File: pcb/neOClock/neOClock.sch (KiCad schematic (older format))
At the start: 46 parts, among them J1 Barrel_Jack, J2 Conn_01x04, J3 Conn_01x04, J4 Conn_01x04, J5 ATECC508A, Q1 2n2222a, Q2 2n2222a, SW1 G71Y, SW2 G71Y, SW3 G71Y, U1 DCDC_LM2596, U2 AMS1117, U3 ESP32_dev_30p, U4 SA15-11GWA, U5 SA15-11GWA, U6 SAA1064, U7 SA15-11GWA, U8 SA15-11GWA

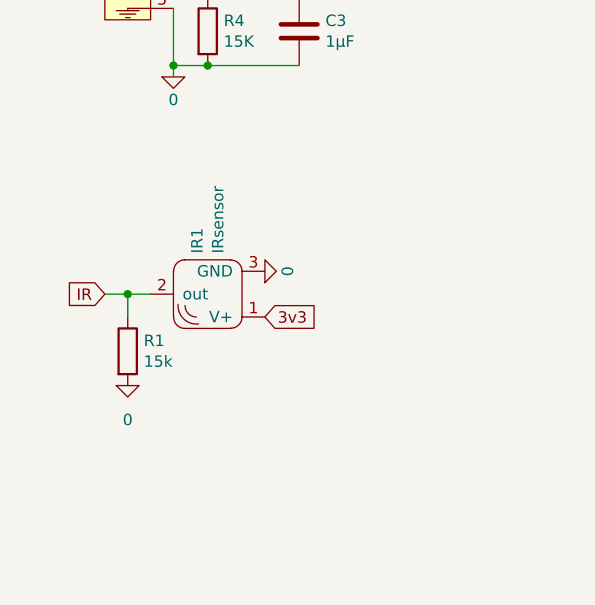
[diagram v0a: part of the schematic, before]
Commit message: update
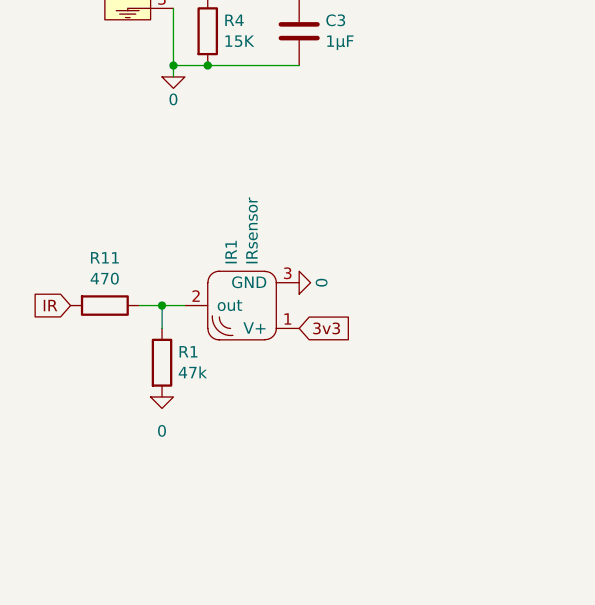
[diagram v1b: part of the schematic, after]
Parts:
- added R11: 470, Resistor_SMD:R_0805_2012Metric_Pad1.20x1.40mm_HandSolder, symbol Device:R
- R1: value 15k -> 47k
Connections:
- net IR: now also R11.2; no longer IR1.2 (out), R1.1
- new net: IR1.2 (out), R1.1, R11.1
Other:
- moved on the sheet: IR1, R1
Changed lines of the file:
@@
 L neosensor_addon:IRsensor IR1
 U 1 1 60A834AB
-P 1300 3700
-F 0 "IR1" V 1346 3522 50  0000 R CNN
-F 1 "IRsensor" V 1255 3522 50  0000 R CNN
-F 2 "neosensor_addon:IRsensor_TH_and_smd" H 1300 3700 50  0001 C CIN
-F 3 "" H 1300 3700 50  0001 C CNN
-	1    1300 3700
+P 1450 3750
+F 0 "IR1" V 1496 3572 50  0000 R CNN
+F 1 "IRsensor" V 1405 3572 50  0000 R CNN
+F 2 "neosensor_addon:IRsensor_TH_and_smd" H 1450 3750 50  0001 C CIN
+F 3 "" H 1450 3750 50  0001 C CNN
+	1    1450 3750
 	-1   0    0    1
 $EndComp
@@
 L pspice:0 #GND0111
 U 1 1 60A9911E
-P 1550 3600
-F 0 "#GND0111" H 1550 3500 50  0001 C CNN
-F 1 "0" H 1550 3500 50  0000 C CNN
-F 2 "" H 1550 3600 50  0001 C CNN
-F 3 "~" H 1550 3600 50  0001 C CNN
-	1    1550 3600
+P 1700 3650
+F 0 "#GND0111" H 1700 3550 50  0001 C CNN
+F 1 "0" H 1700 3550 50  0000 C CNN
+F 2 "" H 1700 3650 50  0001 C CNN
+F 3 "~" H 1700 3650 50  0001 C CNN
+	1    1700 3650
 	0    -1   -1   0
 $EndComp
@@
 Text GLabel 4150 1550 2    50   Input ~ 0
 SCL
-Text GLabel 1550 3800 2    50   Input ~ 0
+Text GLabel 1700 3850 2    50   Input ~ 0
 3v3
 $Comp
@@
 Text GLabel 1750 2350 2    50   Input ~ 0
 Push_3
-Text GLabel 850  3700 0    50   Input ~ 0
+Text GLabel 700  3750 0    50   Input ~ 0
 IR
 Text GLabel 3400 6850 2    50   Input ~ 0
@@
 L Device:R R1
 U 1 1 61383ACF
-P 950 3950
-F 0 "R1" H 1020 3996 50  0000 L CNN
-F 1 "15k" H 1020 3905 50  0000 L CNN
-F 2 "Resistor_SMD:R_0805_2012Metric_Pad1.20x1.40mm_HandSolder" V 880 3950 50  0001 C CNN
-F 3 "~" H 950 3950 50  0001 C CNN
-	1    950  3950
+P 1100 4000
+F 0 "R1" H 1170 4046 50  0000 L CNN
+F 1 "47k" H 1170 3955 50  0000 L CNN
+F 2 "Resistor_SMD:R_0805_2012Metric_Pad1.20x1.40mm_HandSolder" V 1030 4000 50  0001 C CNN
+F 3 "~" H 1100 4000 50  0001 C CNN
+	1    1100 4000
 	1    0    0    -1
 $EndComp
@@
 L pspice:0 #GND0125
 U 1 1 61384771
-P 950 4100
-F 0 "#GND0125" H 950 4000 50  0001 C CNN
-F 1 "0" H 950 3950 50  0000 C CNN
-F 2 "" H 950 4100 50  0001 C CNN
-F 3 "~" H 950 4100 50  0001 C CNN
-	1    950  4100
-	1    0    0    -1
-$EndComp
-Wire Wire Line
-	850  3700 950  3700
-Wire Wire Line
-	950  3700 950  3800
-Connection ~ 950  3700
-Wire Wire Line
-	950  3700 1050 3700
+P 1100 4150
+F 0 "#GND0125" H 1100 4050 50  0001 C CNN
+F 1 "0" H 1100 4000 50  0000 C CNN
+F 2 "" H 1100 4150 50  0001 C CNN
+F 3 "~" H 1100 4150 50  0001 C CNN
+	1    1100 4150
+	1    0    0    -1
+$EndComp
+Wire Wire Line
+	1000 3750 1100 3750
+Wire Wire Line
+	1100 3750 1100 3850
+Connection ~ 1100 3750
+Wire Wire Line
+	1100 3750 1200 3750
 Wire Wire Line
 	3300 6850 3300 6950
@@
 NoConn ~ 8125 1700
 NoConn ~ 10150 1700
+$Comp
+L Device:R R11
+U 1 1 60C98695
+P 850 3750
+F 0 "R11" V 643 3750 50  0000 C CNN
+F 1 "470" V 734 3750 50  0000 C CNN
+F 2 "Resistor_SMD:R_0805_2012Metric_Pad1.20x1.40mm_HandSolder" V 780 3750 50  0001 C CNN
+F 3 "~" H 850 3750 50  0001 C CNN
+	1    850  3750
+	0    1    1    0
+$EndComp
 Wire Bus Line
 	9950 1100 9950 2950

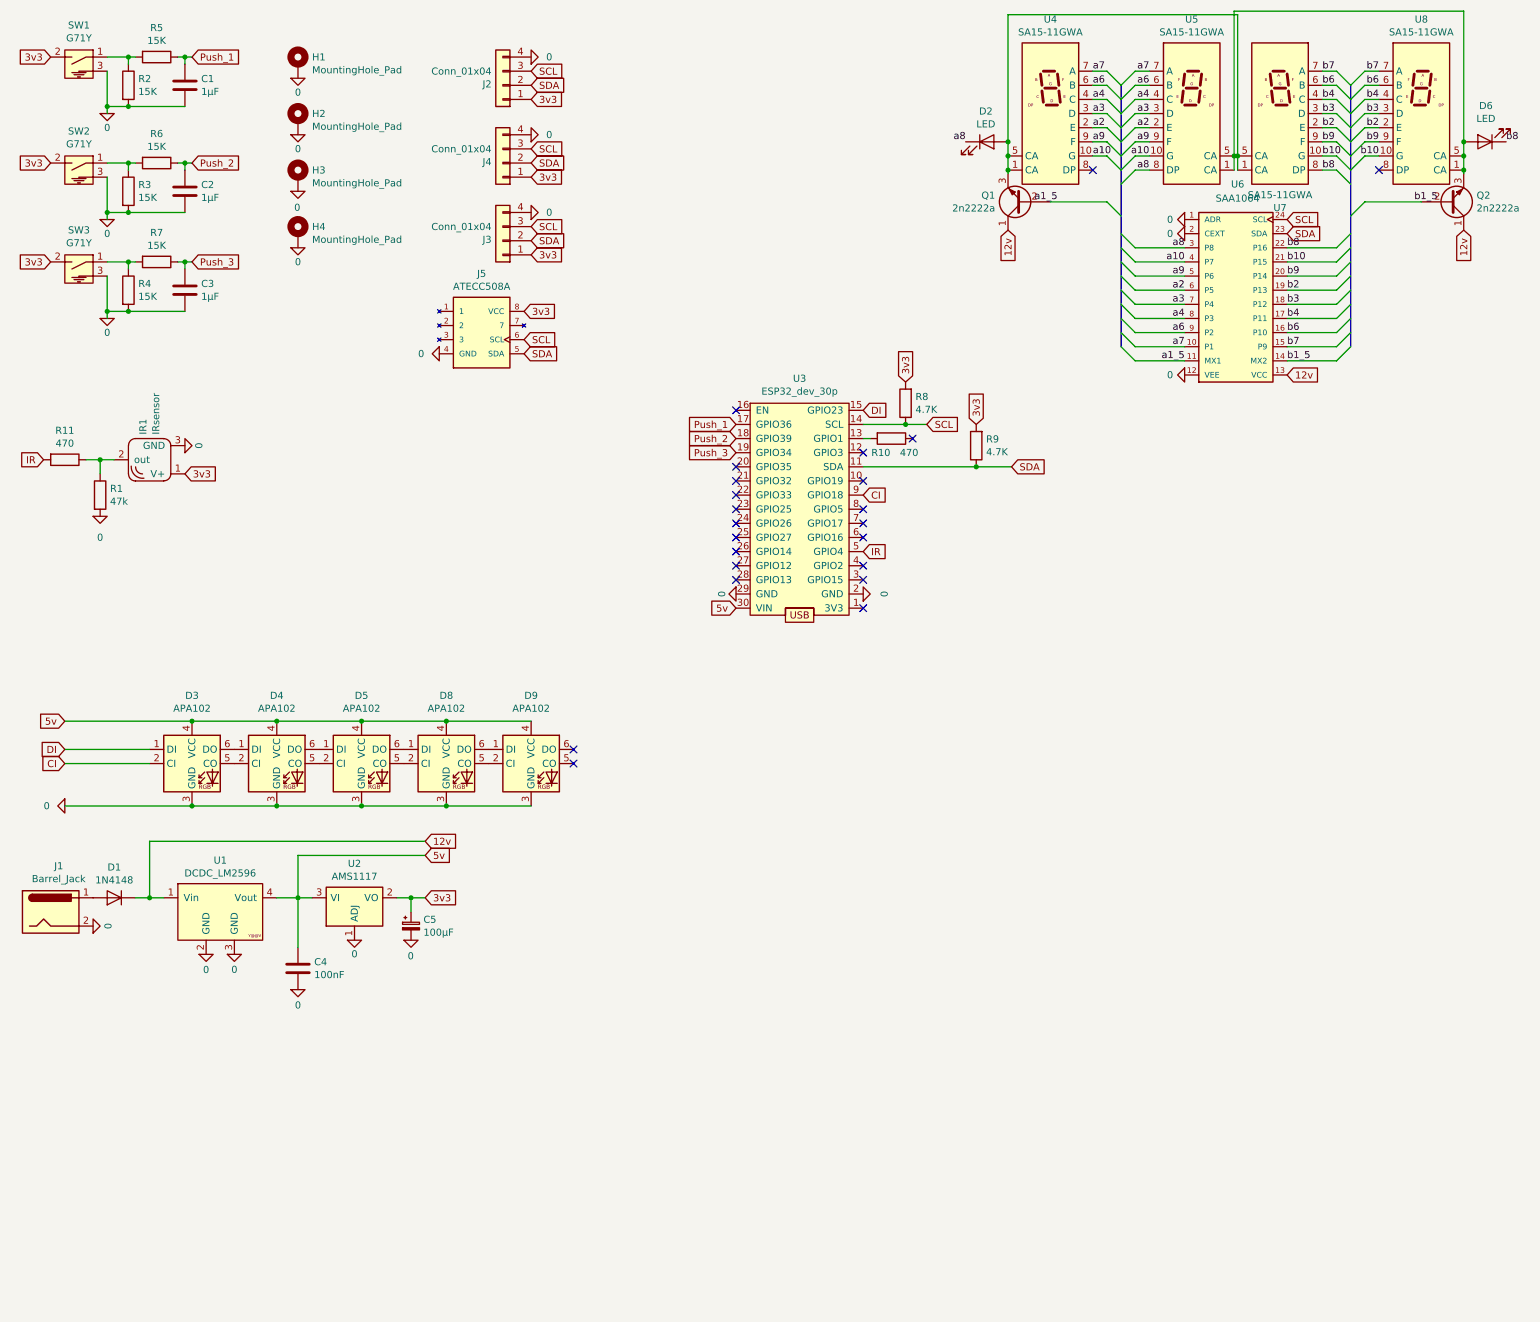
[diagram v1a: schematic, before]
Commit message: update
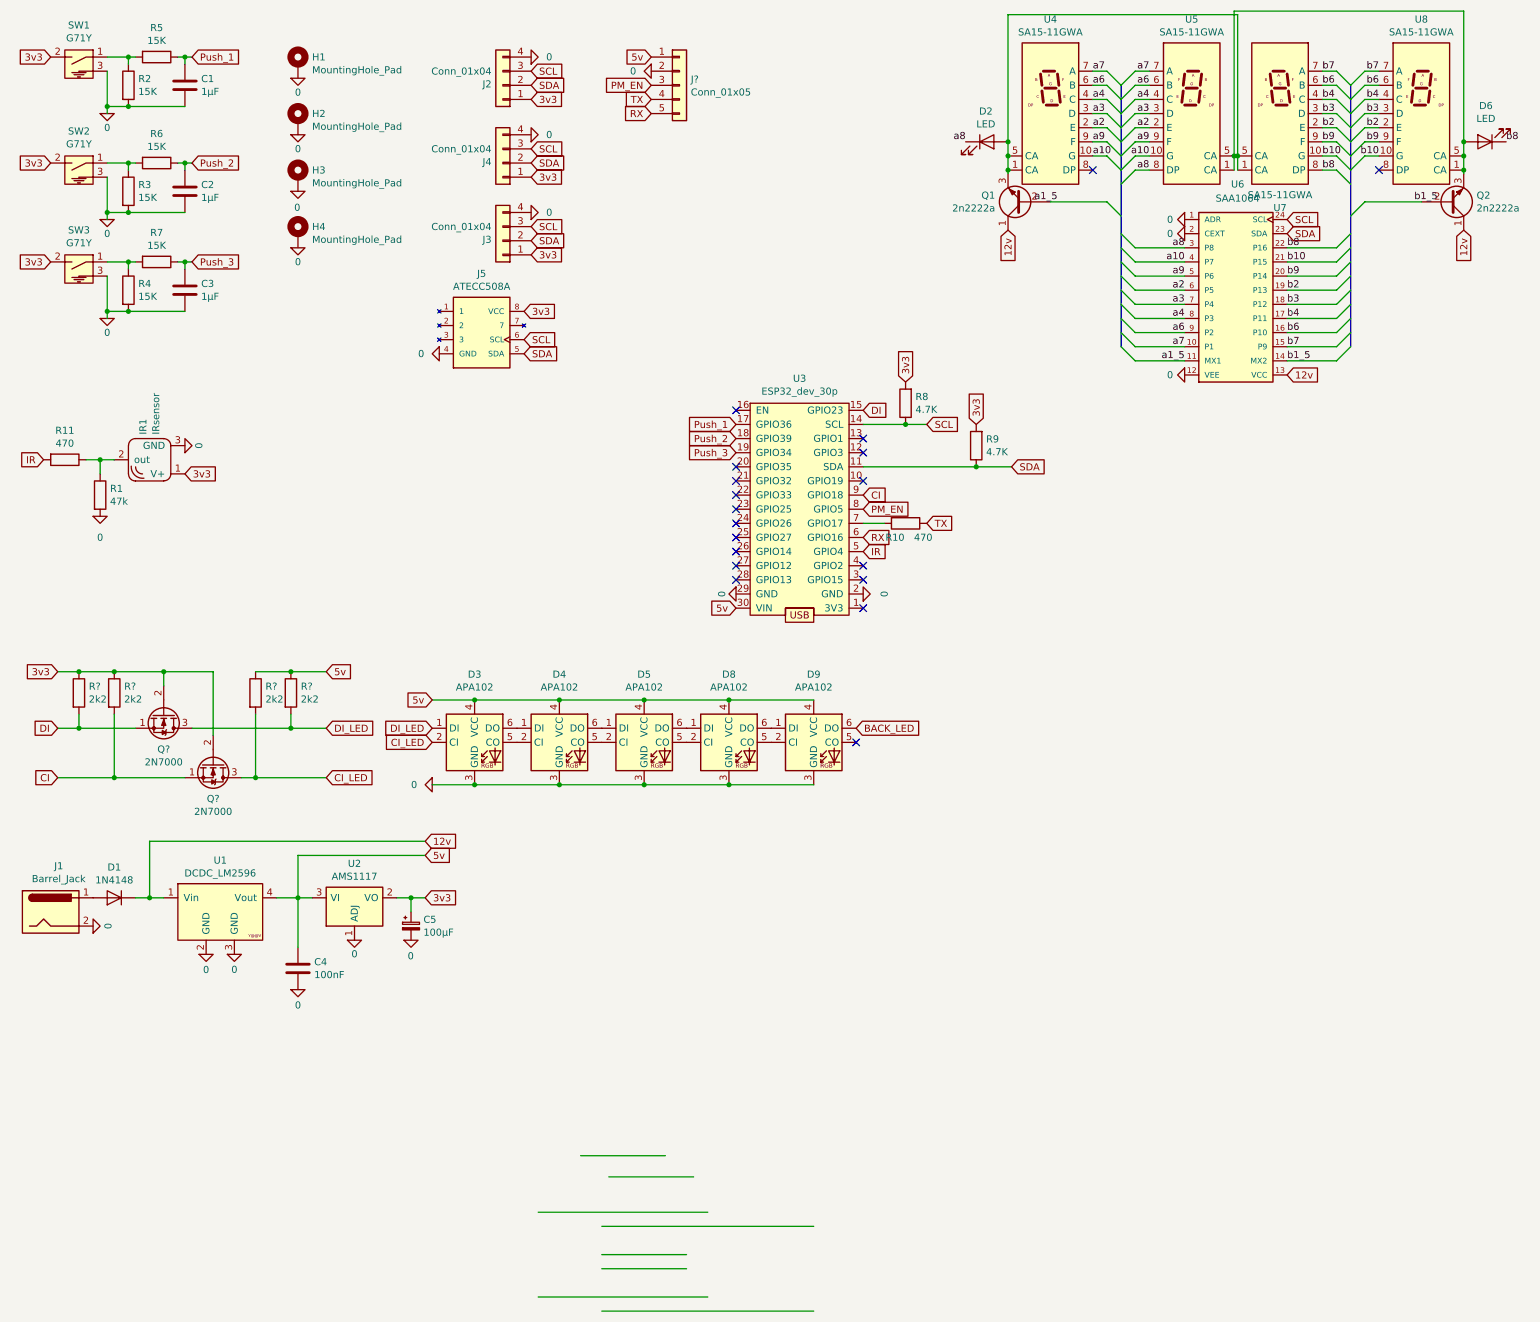
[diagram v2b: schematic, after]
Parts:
- added J?: Conn_01x05, symbol Connector_Generic:Conn_01x05
- added Q? (x2): 2N7000, Package_TO_SOT_THT:TO-92_Inline, symbol Transistor_FET:2N7000
- added R? (x4): 2k2, symbol Device:R
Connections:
- net labels added: BACK_LED, CI_LED, DI_LED, PM_EN, RX, TX
- wire segments 126 -> 152
- no-connect marks 23 -> 19
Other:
- moved on the sheet: D3, D4, D5, D8, D9, R10
